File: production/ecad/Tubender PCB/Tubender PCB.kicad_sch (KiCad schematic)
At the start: 0 parts

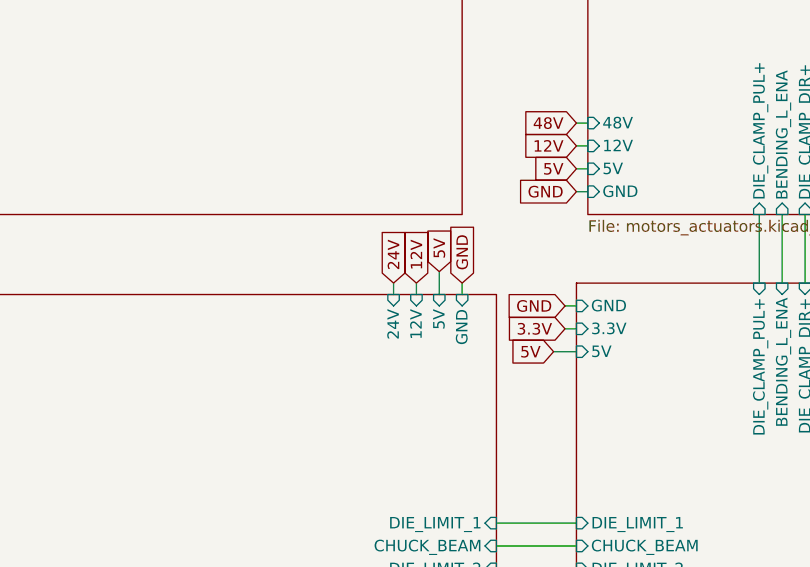
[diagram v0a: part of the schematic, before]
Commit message: sensor updates!
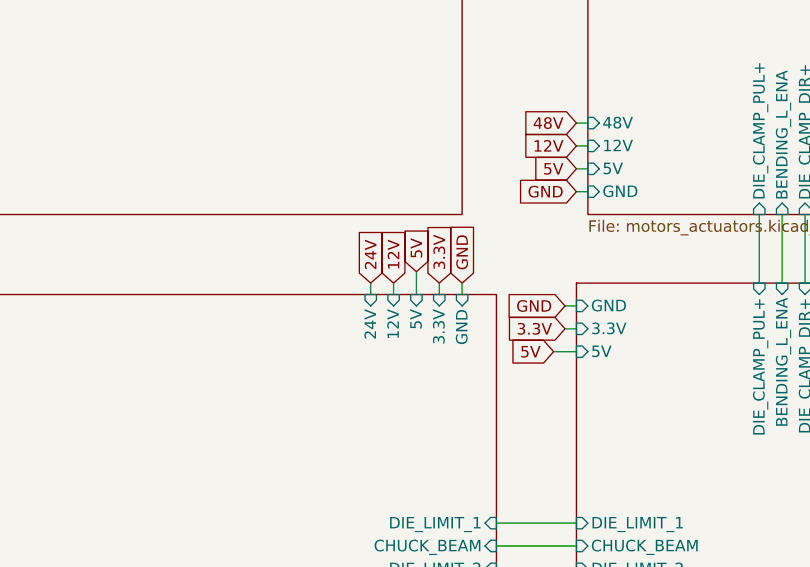
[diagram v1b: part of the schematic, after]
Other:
- sheet SENSORS ports: added 3.3V; removed none
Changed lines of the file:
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@@
 	(wire
 		(pts
-			(xy 90.17 92.71) (xy 90.17 95.25)
+			(xy 87.63 92.71) (xy 87.63 95.25)
 		)
 		(stroke
@@
 	(wire
 		(pts
-			(xy 87.63 93.98) (xy 87.63 95.25)
+			(xy 85.09 93.98) (xy 85.09 95.25)
 		)
 		(stroke
@@
 	(wire
 		(pts
+			(xy 90.17 93.98) (xy 90.17 95.25)
+		)
+		(stroke
+			(width 0)
+			(type default)
+		)
+	)
+	(wire
+		(pts
 			(xy 105.41 83.82) (xy 106.68 83.82)
 		)
@@
 	(wire
 		(pts
-			(xy 85.09 93.98) (xy 85.09 95.25)
+			(xy 82.55 93.98) (xy 82.55 95.25)
 		)
 		(stroke
@@
 	(global_label "3.3V"
 		(shape input)
+		(at 90.17 93.98 90)
+		(fields_autoplaced yes)
+		(effects
+			(font
+				(size 1.27 1.27)
+			)
+			(justify left)
+		)
+		(property "Intersheetrefs" "${INTERSHEET_REFS}"
+			(at 90.17 86.8824 90)
+			(effects
+				(font
+					(size 1.27 1.27)
+				)
+				(justify left)
+				(hide yes)
+			)
+		)
+	)
+	(global_label "3.3V"
+		(shape input)
 		(at 93.98 33.02 0)
 		(fields_autoplaced yes)
@@
 	(global_label "12V"
 		(shape input)
-		(at 87.63 93.98 90)
+		(at 85.09 93.98 90)
 		(fields_autoplaced yes)
 		(effects
@@
 		)
 		(property "Intersheetrefs" "${INTERSHEET_REFS}"
-			(at 87.63 87.4872 90)
+			(at 85.09 87.4872 90)
 			(effects
 				(font
@@
 	(global_label "24V"
 		(shape input)
-		(at 85.09 93.98 90)
+		(at 82.55 93.98 90)
 		(fields_autoplaced yes)
 		(effects
@@
 		)
 		(property "Intersheetrefs" "${INTERSHEET_REFS}"
-			(at 85.09 87.4872 90)
+			(at 82.55 87.4872 90)
 			(effects
 				(font
@@
 	(global_label "5V"
 		(shape input)
-		(at 90.17 92.71 90)
+		(at 87.63 92.71 90)
 		(fields_autoplaced yes)
 		(effects
@@
 		)
 		(property "Intersheetrefs" "${INTERSHEET_REFS}"
-			(at 90.17 87.4267 90)
+			(at 87.63 87.4267 90)
 			(effects
 				(font
@@
 		)
 		(pin "12V" input
+			(at 85.09 95.25 90)
+			(effects
+				(font
+					(size 1.27 1.27)
+				)
+				(justify right)
+			)
+		)
+		(pin "24V" input
+			(at 82.55 95.25 90)
+			(effects
+				(font
+					(size 1.27 1.27)
+				)
+				(justify right)
+			)
+		)
+		(pin "5V" input
 			(at 87.63 95.25 90)
-			(effects
-				(font
-					(size 1.27 1.27)
-				)
-				(justify right)
-			)
-		)
-		(pin "24V" input
-			(at 85.09 95.25 90)
-			(effects
-				(font
-					(size 1.27 1.27)
-				)
-				(justify right)
-			)
-		)
-		(pin "5V" input
-			(at 90.17 95.25 90)
 			(effects
 				(font
@@
 			(effects
 				(font
+					(size 1.27 1.27)
+				)
+				(justify right)
+			)
+		)
+		(pin "3.3V" input
+			(at 90.17 95.25 90)
+			(effects
+				(font
